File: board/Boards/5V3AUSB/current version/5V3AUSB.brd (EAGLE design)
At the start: 36.8 x 51.7 mm, 18 parts

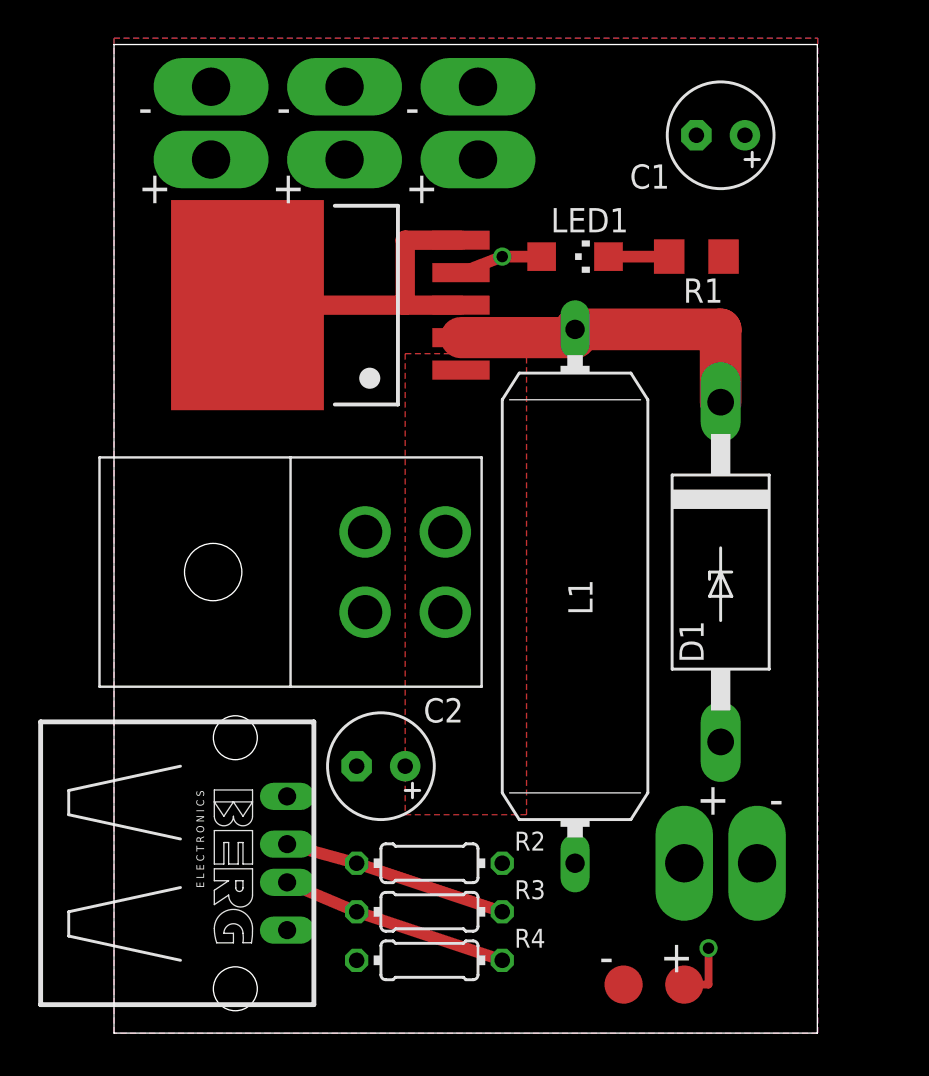
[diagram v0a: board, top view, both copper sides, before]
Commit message: updates to 5V 3A board
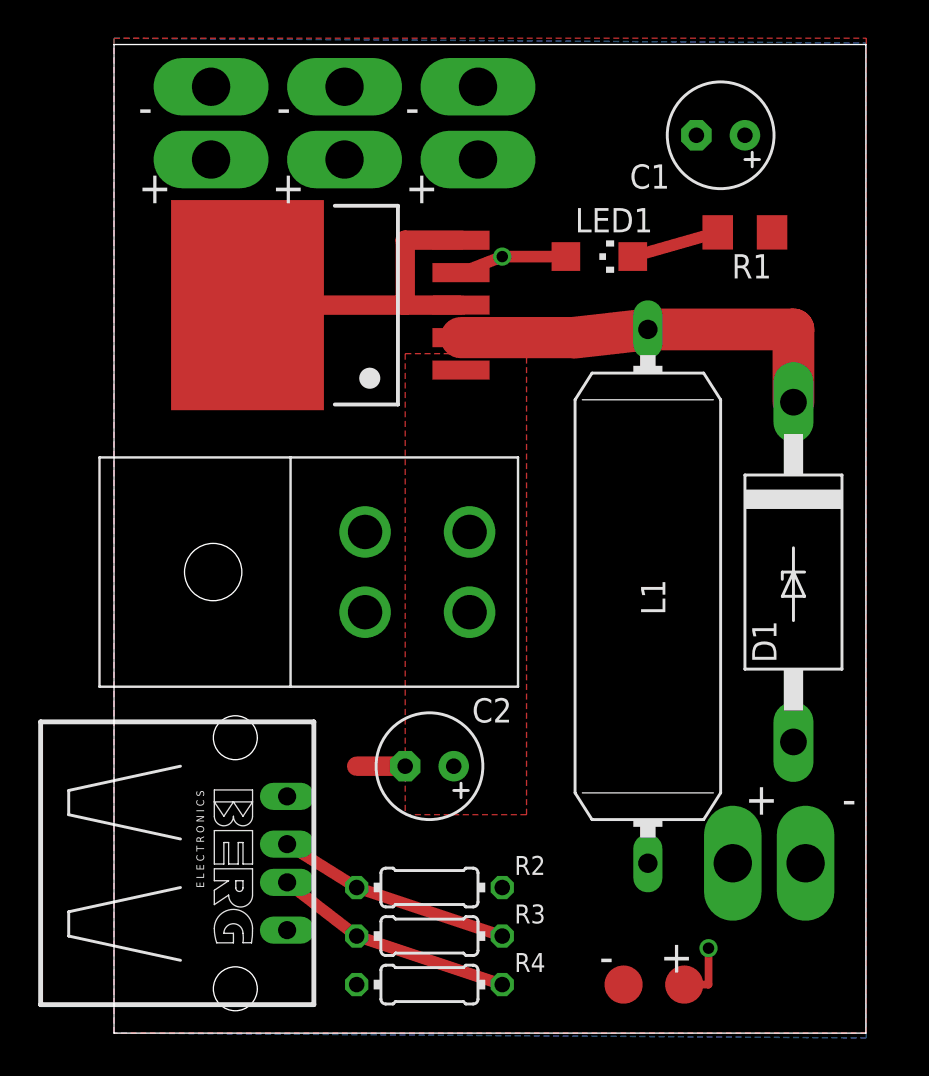
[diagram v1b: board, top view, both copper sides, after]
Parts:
- moved D1 3.81 mm to (35.6, 24.1)
- moved L1 3.81 mm to (27.9, 22.9)
- moved R1 2.84 mm to (33.0, 41.9)
- moved C2 2.54 mm to (16.5, 14.0)
- moved TP3 2.54 mm to (34.3, 8.89)
- moved R2 1.27 mm to (16.5, 7.62)
- moved R4 1.27 mm to (16.5, 2.54)
- moved LED1 1.27 mm to (25.4, 40.6)
- moved R3 1.27 mm to (16.5, 5.08)
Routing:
- net N$2: track 17.8 -> 21.2 mm
- net GND: track 17.5 -> 20.0 mm
- net N$5: track 3.18 -> 4.63 mm
- net N$3: track 7.55 -> 8.82 mm
- net N$6: track 12.0 -> 12.6 mm
- net N$7: track 11.8 -> 12.3 mm
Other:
- board size 36.8 x 51.7 mm -> 39.4 x 51.7 mm
- board text added: "5V 3A USB Power V1.1 C.G & D.K hitchBOT Dec 2014"
- board text removed: "5V 3A USB Power V1.0 C.G & D.K hitchBOT August 2014"
